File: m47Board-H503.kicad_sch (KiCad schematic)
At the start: 42 parts, among them J1 USB_C_Receptacle_USB2.0_16P, J3 Conn_01x15_Pin, J4 Conn_01x10_Pin, J5 Conn_01x15_Pin, SW1 SW_Push, SW2 SW_Push, SW3 SW_Push, U1 AP2114H-3.3TRG1, U2 STM32H503CBTx, U3 USBLC6-2SC6, Y1 CX3225FB16000F0FZZH1 16MHz, Y2 ABS07-32.768KHZ-T

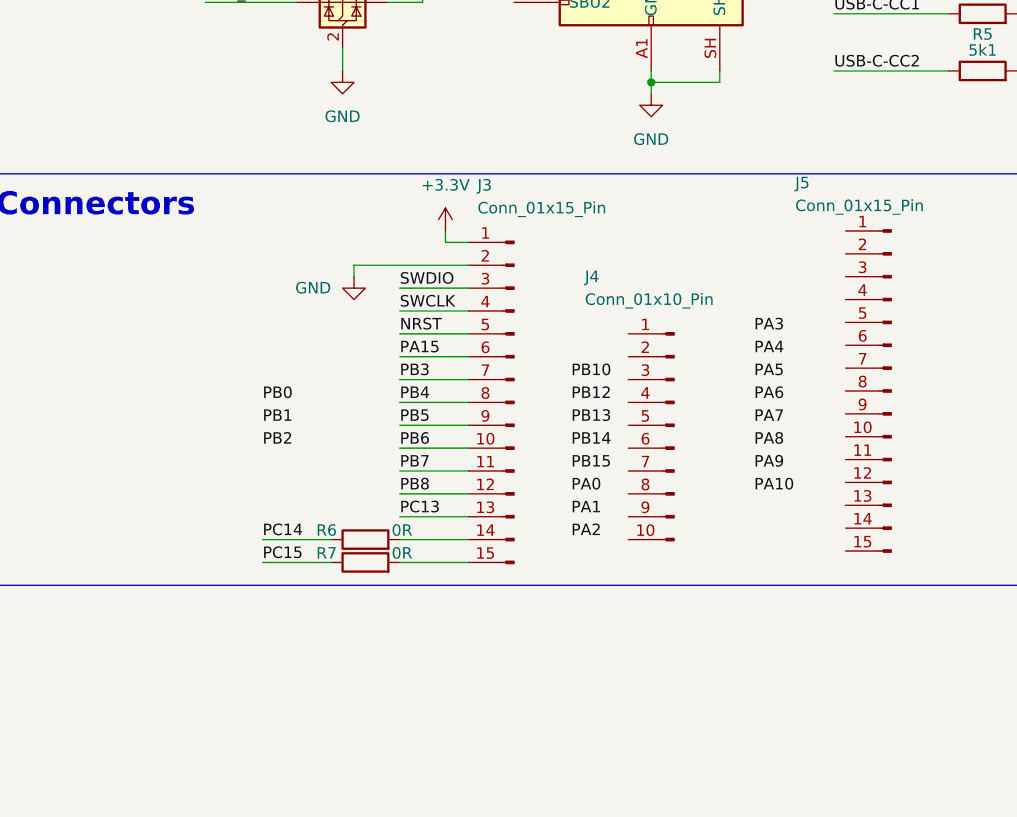
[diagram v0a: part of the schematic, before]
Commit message: Route tracks
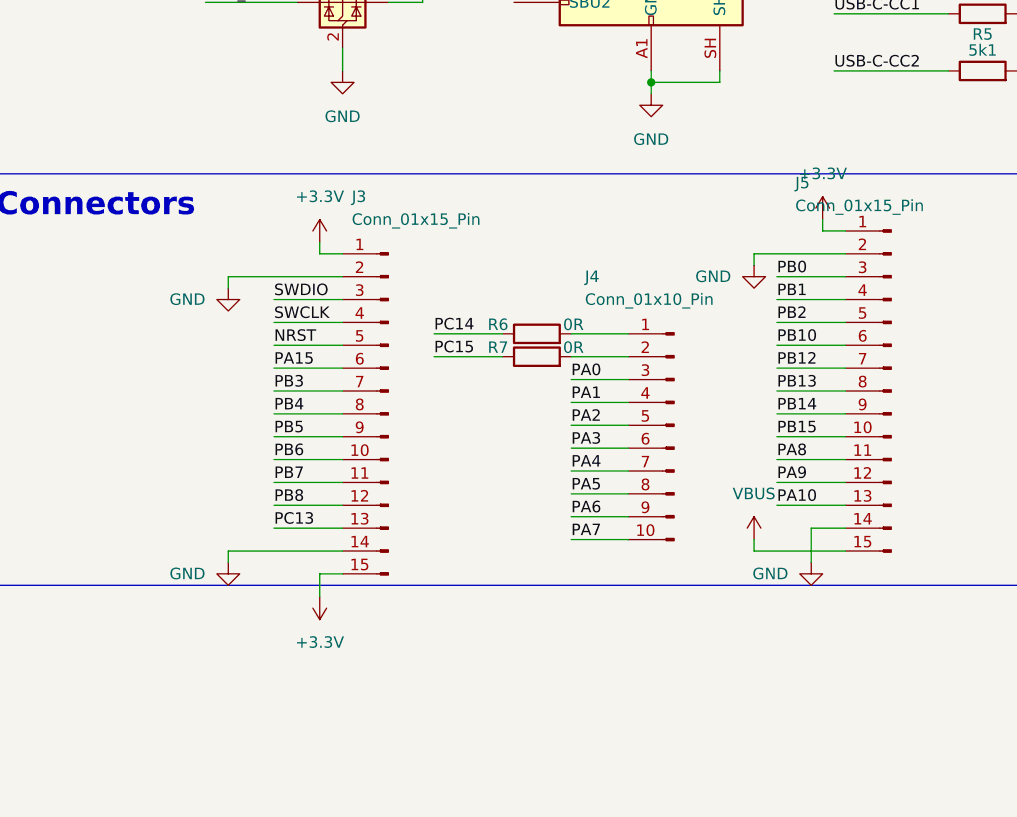
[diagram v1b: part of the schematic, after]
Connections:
- net +3.3V: now also J3.15 (Pin_15), J5.1 (Pin_1)
- net GND: now also J3.14 (Pin_14), J5.14 (Pin_14), J5.2 (Pin_2)
- net PA0: now also J4.3 (Pin_3)
- net PA1: now also J4.4 (Pin_4)
- net PA10: now also J5.13 (Pin_13)
- net PA2: now also J4.5 (Pin_5)
- net PA3: now also J4.6 (Pin_6)
- net PA4: now also J4.7 (Pin_7)
- net PA5: now also J4.8 (Pin_8)
- net PA6: now also J4.9 (Pin_9)
- net PA7: now also J4.10 (Pin_10)
- net PA8: now also J5.11 (Pin_11)
- net PA9: now also J5.12 (Pin_12)
- net PB0: now also J5.3 (Pin_3)
- net PB1: now also J5.4 (Pin_4)
- net PB10: now also J5.6 (Pin_6)
- net PB12: now also J5.7 (Pin_7)
- net PB13: now also J5.8 (Pin_8)
- net PB14: now also J5.9 (Pin_9)
- net PB15: now also J5.10 (Pin_10)
- net PB2: now also J5.5 (Pin_5)
- net VBUS: now also J5.15 (Pin_15)
- net at R7.2: now also J4.2 (Pin_2); no longer J3.15 (Pin_15)
- net at J4.1 (Pin_1): now also R6.2
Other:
- moved on the sheet: J3, R6, R7
